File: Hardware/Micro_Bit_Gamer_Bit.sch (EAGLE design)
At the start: 21 parts, among them J1 I2C, U1 micro:bit

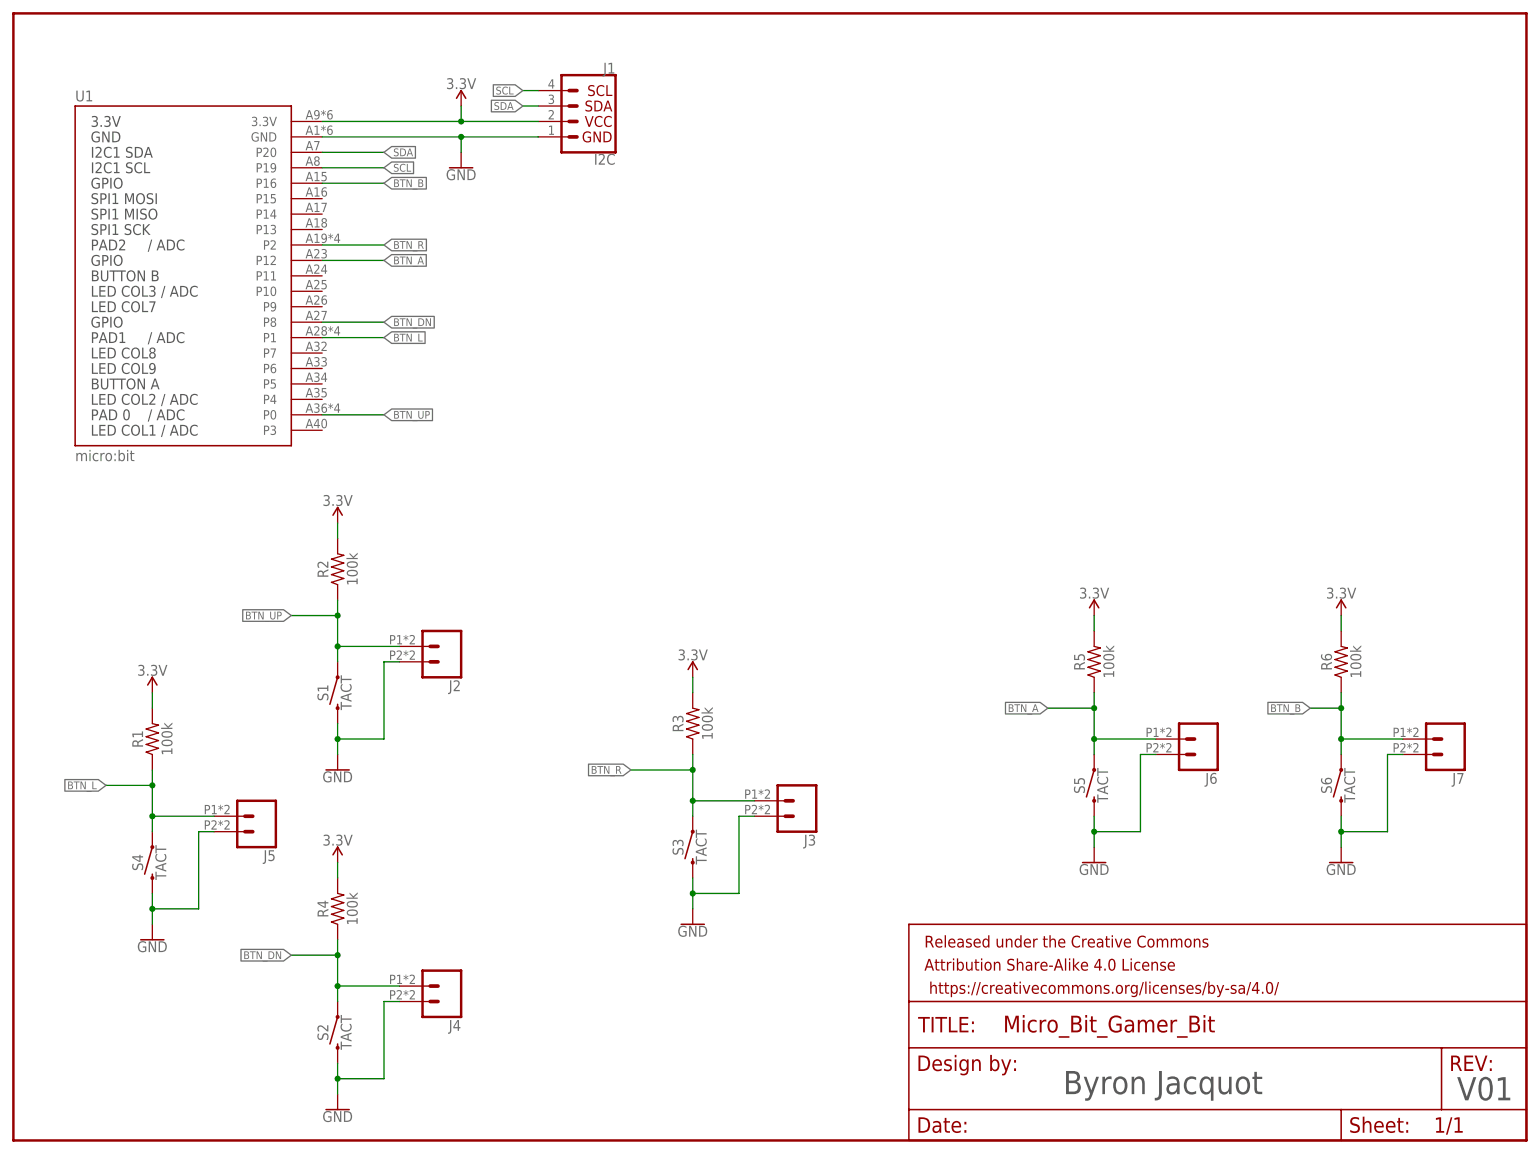
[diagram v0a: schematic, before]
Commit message: Board routed, ready for review.
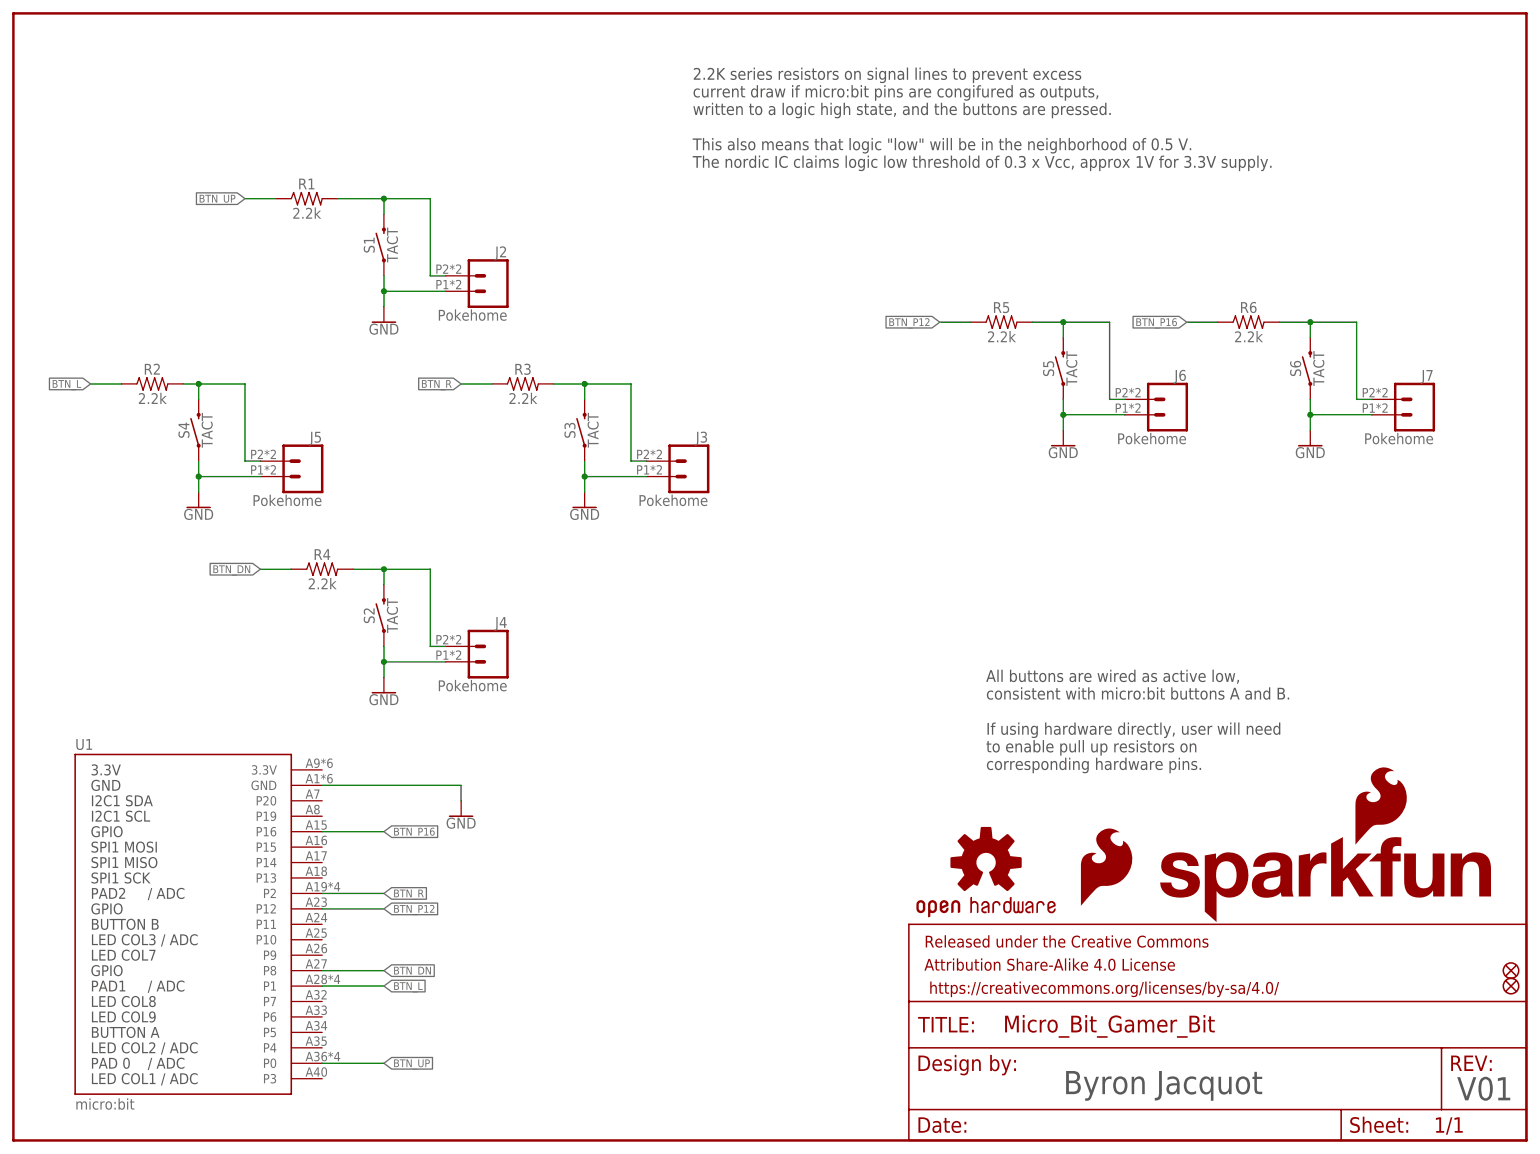
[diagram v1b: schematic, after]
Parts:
- removed J1: I2C, SparkFun-Connectors:I2C_STANDARD_NO_SILK
- added FD1, FD2: FIDUCIALUFIDUCIAL, SparkFun-Aesthetics:FIDUCIALUFIDUCIAL
- added LOGO1: SFE_LOGO_FLAME.5_INCH, SparkFun-Aesthetics:SFE_LOGO_FLAME.5_INCH
- added LOGO2: OSHW-LOGOS, SparkFun-Aesthetics:OSHW-LOGOS
- added LOGO3: SFE_LOGO_NAME_FLAME.3_INCH, SparkFun-Aesthetics:SFE_LOGO_NAME_FLAME.3_INCH
- J2, J3, J4, J5, J6, J7: value (none) -> Pokehome
- R1, R2, R3, R4, R5, R6: value 100k -> 2.2k; device SparkFun-Resistors:100KOHM-0603-1/10W-1% -> SparkFun-Resistors:2.2KOHM-0603-1/10W-1%
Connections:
- removed net 3.3V: J1.2, R1.2, R2.2, R3.2, R4.2, R5.2, R6.2, U1.3.3V
- removed net BTN_A: J6.1, R5.1, S5.1, U1.P12
- removed net BTN_B: J7.1, R6.1, S6.1, U1.P16
- removed net SCL: J1.4, U1.P19
- removed net SDA: J1.3, U1.P20
- new net BTN_P12: R5.1, U1.P12
- new net BTN_P16: R6.1, U1.P16
- new net N$1: J2.2, R1.2, S1.2
- new net N$2: J5.2, R2.2, S4.2
- new net N$3: J4.2, R4.2, S2.2
- new net N$4: J3.2, R3.2, S3.2
- new net N$5: J7.2, R6.2, S6.2
- new net N$80: J6.2, R5.2, S5.2
- net BTN_DN: no longer J4.1, S2.1
- net BTN_L: now also R2.1; no longer J5.1, R1.1, S4.1
- net BTN_R: no longer J3.1, S3.1
- net BTN_UP: now also R1.1; no longer J2.1, R2.1, S1.1
- net GND: now also J2.1, J3.1, J4.1, J5.1, J6.1, J7.1, S1.1, S2.1, S3.1, S4.1, S5.1, S6.1; no longer J1.1, J2.2, J3.2, J4.2, J5.2, J6.2, J7.2, S1.2, S2.2, S3.2, S4.2, S5.2, S6.2
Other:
- note added: "2.2K series resistors on signal lines to prevent excess current draw if micro:bit pins are congifured as outputs, written to a logic high state, and the buttons are pressed. This also means that logic "low" will be in the neighborhood of 0.5 V. The nordic IC claims logic low threshold of 0.3 x Vcc, approx 1V for 3.3V supply."
- note added: "All buttons are wired as active low, consistent with micro:bit buttons A and B. If using hardware directly, user will need to enable pull up resistors on corresponding hardware pins."
- moved on the sheet: J2, J3, J4, J5, J6, J7, R1, R2, R3, R4, R5, R6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
